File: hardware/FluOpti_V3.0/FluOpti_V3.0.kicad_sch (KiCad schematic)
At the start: 115 parts, among them J1 HDR-2x1, J10 HDR-2x1, J10 USB_B_Micro, J11 LED_1, J12 LED_3, J13 HDR-4x1, J14 HDR-2x1, J15 TP-PWR_IN, J16 HDR-2x1, J17 HDR-2x1, J18 HDR-2x1, J19 LED_2, J20 LED_4, J3 HDR-2x1, J4 HDR-2x1, J5 HDR-2x1, J6 HDR-2x1, J7 TP-PWR_IN, J8 TP-5V, J9 TP-3.3V, Q1 Q_PMOS_GSD, Q3 NPN, Q4 NPN, Q4 Q_Dual_NPN_NPN_BRT_E1B1C2E2B2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, Q5 NPN, Q6 NPN, Q7 NPN, Q8 NPN, SW2 SW_DIP_x02, SW3 SW_DIP_x02, U10 ADS1115IDGS, U10 ESP32-WROOM-32D, U11 AD5659R, U2 AP2112K-3.3TRG1, U3 XL6008, U4 MT3608, U7 TLC272, U8 TLC272, U9 CH340C, U9 TLC272

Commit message: actualizacion_PCB
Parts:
- removed C19: 100n, Capacitor_SMD:C_0603_1608Metric, symbol IoWLabs:C
- removed C20: 10u, Capacitor_SMD:C_0805_2012Metric, symbol IoWLabs:C
- removed JP2: Jumper_2_Open, Jumper:SolderJumper-2_P1.3mm_Open_RoundedPad1.0x1.5mm, symbol Jumper:Jumper_2_Open
- removed R16: 2k, Resistor_SMD:R_0603_1608Metric, symbol Device:R
- removed R17, R18, R19: 10k, Resistor_SMD:R_0603_1608Metric, symbol Device:R
- removed U11: AD5659R, Package_SO:TSSOP-16_4.4x5mm_P0.65mm, symbol IoWLabs:AD5669R
- added C24, C26: 100n, Capacitor_SMD:C_0603_1608Metric, symbol IoWLabs:C
- added C25, C27: 10u, Capacitor_SMD:C_0805_2012Metric, symbol IoWLabs:C
- added JP4, JP5, JP6, JP7, JP8, JP9: SolderJumper_3_Open, Jumper:SolderJumper-3_P1.3mm_Open_RoundedPad1.0x1.5mm, symbol Jumper:SolderJumper_3_Open
- added Q10, Q9: Q_NMOS_GSD, Package_TO_SOT_SMD:SOT-23, symbol Device:Q_NMOS_GSD
- added R37, R41, R43, R47: 2k, Resistor_SMD:R_0603_1608Metric, symbol Device:R
- added R38, R39, R40, R42, R44, R45, R46, R48, R49, R50, R51, R52: 10k, Resistor_SMD:R_0603_1608Metric, symbol Device:R
- added U12, U13: ~, Package_SO:TSSOP-14_4.4x5mm_P0.65mm, symbol IoWLabs:AD5625R
- R24, R25, R26, R32, R33, R34: footprint IoWLabs:TO-263-3 TAB 3 -> IoWLabs:D2PAK
- R4: value 10 -> 1k
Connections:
- net 3.3V: now also Q10.1 (G), Q9.1 (G), R49.1, R51.1
- net 5V: now also C24.1, C25.1, C26.1, C27.1, JP8.3 (B), JP9.3 (B), R37.2, R39.2, R40.2, R41.2, R43.2, R45.2, R46.2, R47.2, R50.1, R52.1, U12.3 (VDD), U12.7 (VREF), U13.3 (VDD), U13.7 (VREF)
- net GND: now also C24.2, C25.2, C26.2, C27.2, JP8.1 (A), JP9.1 (A), R38.2, R42.2, R44.2, R48.2, U12.12 (GND), U13.12 (GND)
- net SCL: now also Q9.2 (S), R51.2
- net SDA: now also Q10.2 (S), R49.2
- net V_H_1: now also U13.11 (Vout_B)
- net V_H_2: now also U13.4 (Vout_A)
- net V_LED_1: now also U12.4 (Vout_A)
- net V_LED_2: now also JP6.2 (C), U12.11 (Vout_B), U12.8 (ADDR2)
- net V_LED_3: now also U12.5 (Vout_C)
- net V_LED_4: now also U12.10 (Vout_D)
- new net: JP4.1 (A), R38.1
- new net: JP4.2 (C), U13.2 (ADDR1)
- new net: JP4.3 (B), R37.1
- new net: JP9.2 (C), U12.6 (POR)
- new net: JP5.3 (B), R41.1
- new net: JP7.1 (A), R47.1
- new net: JP6.1 (A), R43.1
- new net: JP5.2 (C), U12.2 (ADDR1)
- new net: JP8.2 (C), U13.6 (POR)
- new net: JP7.3 (B), R48.1
- new net: JP5.1 (A), R42.1
- new net: JP7.2 (C), U13.8 (ADDR2)
- new net: JP6.3 (B), R44.1
- new net SCL_5V: Q9.3 (D), R39.1, R45.1, R52.2, U12.14 (SCL), U13.14 (SCL)
- new net SDA_5V: Q10.3 (D), R40.1, R46.1, R50.2, U12.13 (SDA), U13.13 (SDA)
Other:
- note added: "Conversor Logico"
- note added: "I2C DAC 4 channels"
- note removed: "I2C DAC"
- moved on the sheet: C19, J10, J11, J12, J13, J15, J16, J17, J18, J19, J20, J5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

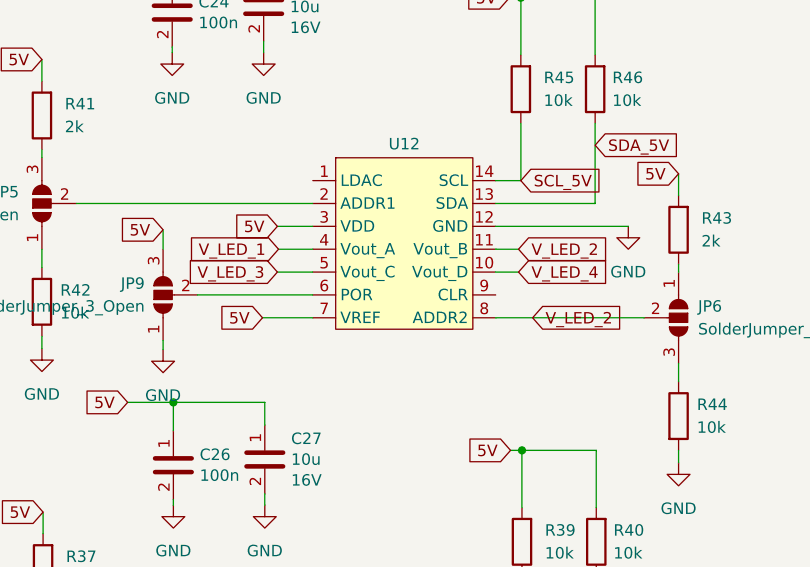
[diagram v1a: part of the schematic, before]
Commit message: PCB
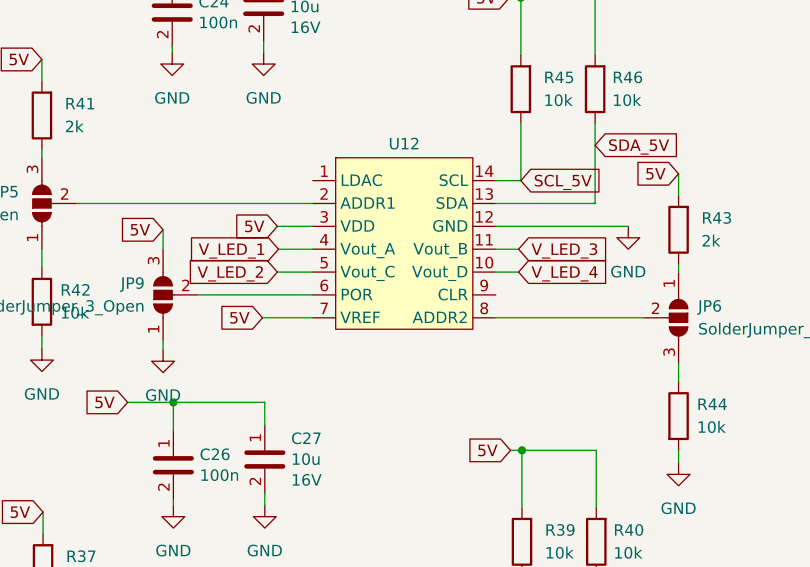
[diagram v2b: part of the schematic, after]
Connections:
- net V_LED_2: now also U12.5 (Vout_C); no longer JP6.2 (C), U12.11 (Vout_B), U12.8 (ADDR2)
- net V_LED_3: now also U12.11 (Vout_B); no longer U12.5 (Vout_C)
- new net: JP6.2 (C), U12.8 (ADDR2)
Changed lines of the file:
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@@
 	(wire
 		(pts
-			(xy 538.353 73.533) (xy 554.863 73.533)
-		)
-		(stroke
-			(width 0)
-			(type default)
-		)
-	)
-	(wire
-		(pts
 			(xy 538.48 123.825) (xy 554.99 123.825)
 		)
@@
 	(wire
 		(pts
+			(xy 538.353 73.533) (xy 554.863 73.533)
+		)
+		(stroke
+			(width 0)
+			(type default)
+		)
+	)
+	(wire
+		(pts
 			(xy 518.16 118.745) (xy 514.223 118.745)
 		)
@@
 		)
 	)
-	(global_label "V_LED_3"
-		(shape input)
-		(at 514.096 68.453 180)
-		(fields_autoplaced yes)
-		(effects
-			(font
-				(size 1.27 1.27)
-			)
-			(justify right)
-		)
-		(property "Intersheetrefs" "${INTERSHEET_REFS}"
-			(at 503.4304 68.453 0)
-			(effects
-				(font
-					(size 1.27 1.27)
-				)
-				(justify right)
-				(hide yes)
-			)
-		)
-	)
 	(global_label "+12V"
 		(shape input)
@@
 		)
 	)
-	(global_label "V_LED_2"
-		(shape input)
-		(at 540.893 65.913 0)
-		(fields_autoplaced yes)
-		(effects
-			(font
-				(size 1.27 1.27)
-			)
-			(justify left)
-		)
-		(property "Intersheetrefs" "${INTERSHEET_REFS}"
-			(at 551.5586 65.913 0)
-			(effects
-				(font
-					(size 1.27 1.27)
-				)
-				(justify left)
-				(hide yes)
-			)
-		)
-	)
 	(global_label "VCC_LED_3"
 		(shape input)
@@
 		)
 	)
-	(global_label "V_LED_2"
+	(global_label "SCL"
 		(shape input)
-		(at 542.4552 73.533 0)
+		(at 360.045 47.625 0)
 		(fields_autoplaced yes)
 		(effects
@@
 		)
 		(property "Intersheetrefs" "${INTERSHEET_REFS}"
-			(at 553.1208 73.533 0)
+			(at 366.5378 47.625 0)
 			(effects
 				(font
@@
 		)
 	)
-	(global_label "SCL"
+	(global_label "EN_V"
 		(shape input)
-		(at 360.045 47.625 0)
+		(at 248.92 51.435 0)
 		(fields_autoplaced yes)
 		(effects
@@
 		)
 		(property "Intersheetrefs" "${INTERSHEET_REFS}"
-			(at 366.5378 47.625 0)
+			(at 256.3615 51.435 0)
 			(effects
 				(font
@@
 		)
 	)
-	(global_label "EN_V"
+	(global_label "I_H1"
 		(shape input)
-		(at 248.92 51.435 0)
+		(at 415.544 198.12 180)
 		(fields_autoplaced yes)
 		(effects
@@
 				(size 1.27 1.27)
 			)
-			(justify left)
+			(justify right)
 		)
 		(property "Intersheetrefs" "${INTERSHEET_REFS}"
-			(at 256.3615 51.435 0)
+			(at 408.5258 198.12 0)
 			(effects
 				(font
 					(size 1.27 1.27)
 				)
-				(justify left)
+				(justify right)
 				(hide yes)
 			)
 		)
 	)
-	(global_label "I_H1"
+	(global_label "VCC_H1"
 		(shape input)
-		(at 415.544 198.12 180)
+		(at 449.199 146.05 180)
 		(fields_autoplaced yes)
 		(effects
@@
 		)
 		(property "Intersheetrefs" "${INTERSHEET_REFS}"
-			(at 408.5258 198.12 0)
+			(at 439.0776 146.05 0)
 			(effects
 				(font
@@
 		)
 	)
-	(global_label "VCC_H1"
+	(global_label "V_H_1"
 		(shape input)
-		(at 449.199 146.05 180)
+		(at 296.037 209.804 180)
 		(fields_autoplaced yes)
 		(effects
@@
 		)
 		(property "Intersheetrefs" "${INTERSHEET_REFS}"
-			(at 439.0776 146.05 0)
+			(at 287.488 209.804 0)
 			(effects
 				(font
@@
 		)
 	)
-	(global_label "V_H_1"
+	(global_label "V_LED_2"
 		(shape input)
-		(at 296.037 209.804 180)
+		(at 514.096 68.453 180)
 		(fields_autoplaced yes)
 		(effects
@@
 		)
 		(property "Intersheetrefs" "${INTERSHEET_REFS}"
-			(at 287.488 209.804 0)
+			(at 503.4304 68.453 0)
 			(effects
 				(font
@@
 				(hide yes)
 			)
+		)
+	)
+	(global_label "V_LED_3"
+		(shape input)
+		(at 540.893 65.913 0)
+		(fields_autoplaced yes)
+		(effects
+			(font
+				(size 1.27 1.27)
+			)
+			(justify left)
+		)
+		(property "Intersheetrefs" "${INTERSHEET_REFS}"
+			(at 551.5586 65.913 0)
+			(effects
+				(font
+					(size 1.27 1.27)
+				)
+				(justify left)
+				(hide yes)
+			)
